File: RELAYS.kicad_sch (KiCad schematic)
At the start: 19 parts, among them J300 DOOR_OUTPUT, J301 Panic_Button, J302 Door_Sensor, K300 HF49FD/005-1H12T, Q300 MMBT3904

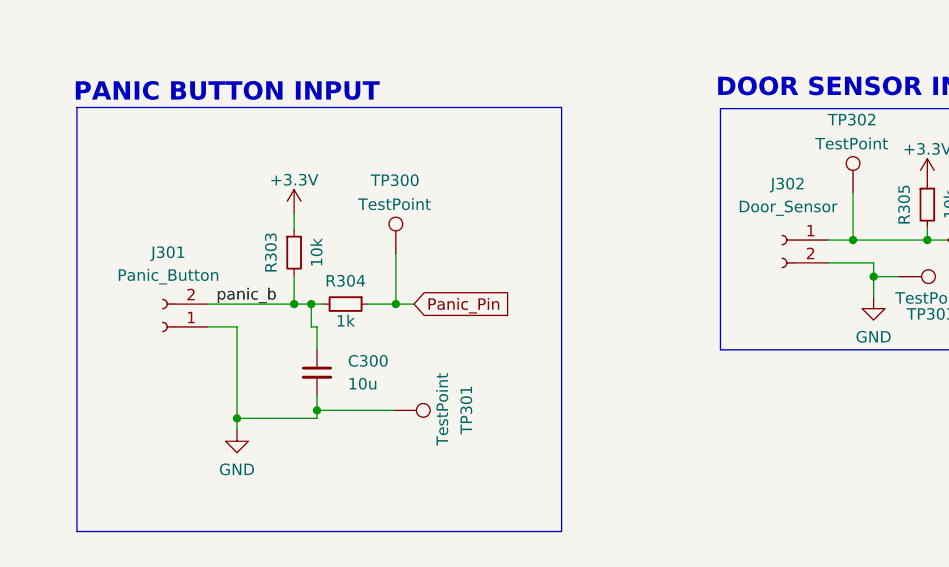
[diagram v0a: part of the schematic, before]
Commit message: version validada
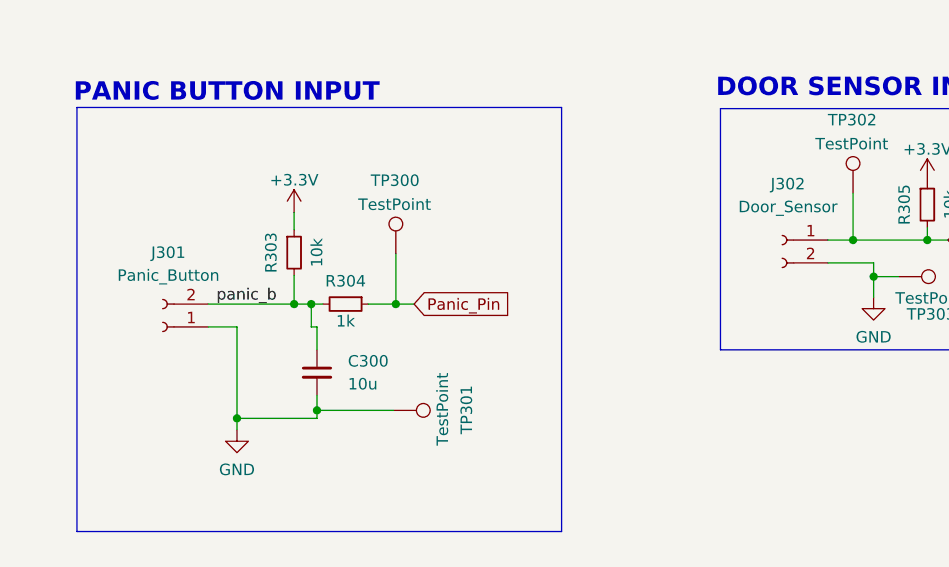
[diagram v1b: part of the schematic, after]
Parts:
- K300: symbol HF49FD_005-1H12T:HF49FD/005-1H12T -> HF49FD_005-1H12T:HF49FD/005-1H12T
